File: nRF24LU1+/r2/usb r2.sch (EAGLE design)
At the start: 19 parts, among them IC2 NRF24L01SMD

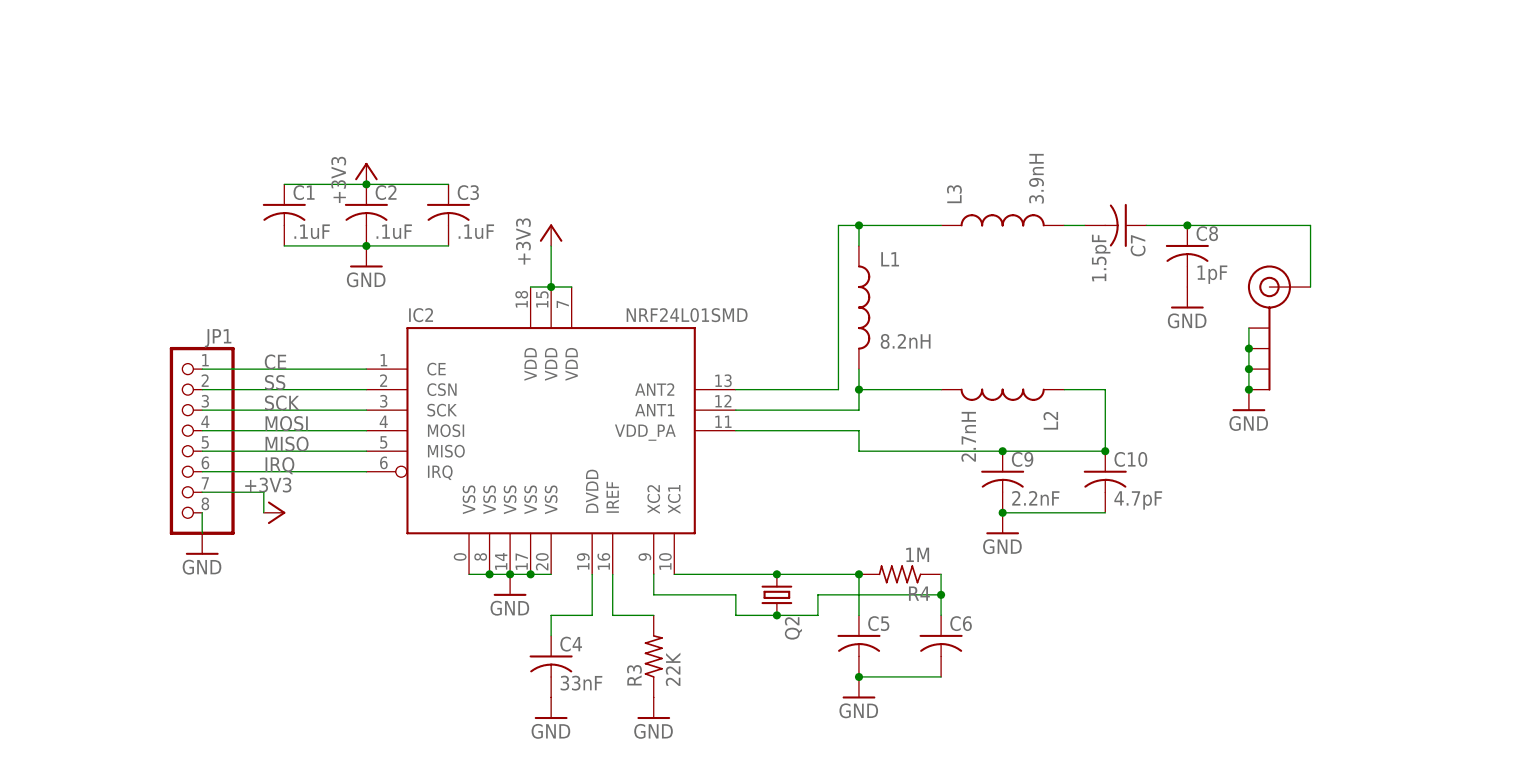
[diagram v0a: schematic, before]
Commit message: cleaning up, added a revised usb breakout
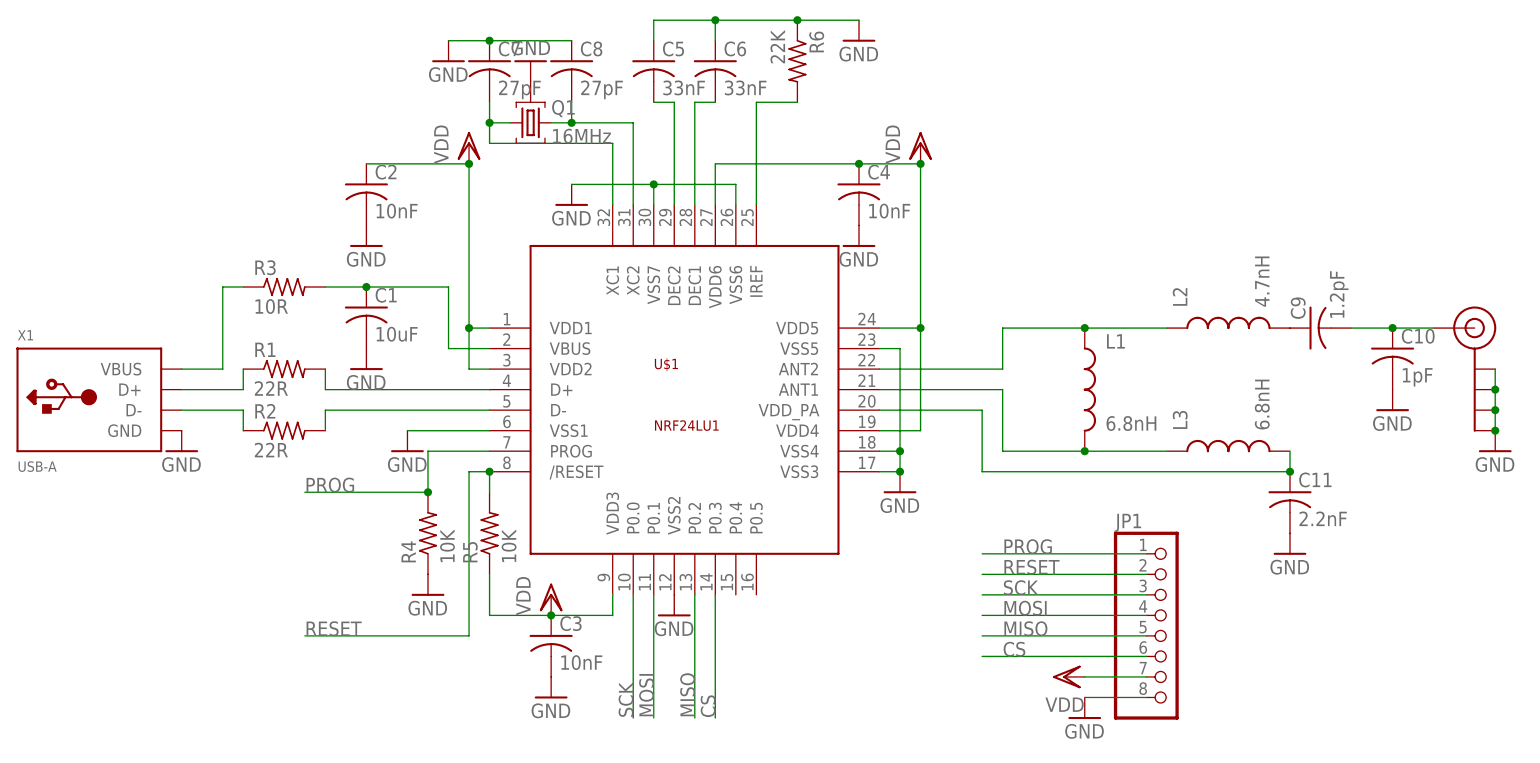
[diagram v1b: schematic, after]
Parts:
- removed IC2: NRF24L01SMD, SparkFun:NRF24L01SMD
- removed Q2: (no value), crystal:CRYSTALHC49U-V
- added C11: 2.2nF, adafruit:C-USC0402
- added Q1: 16MHz, crystal:TSX-3225
- added R1, R2: 22R, adafruit:R-US_R0402
- added R5: 10K, adafruit:R-US_R0402
- added R6: 22K, adafruit:R-US_R0402
- added U$1: NRF24LU1, SparkFun:NRF24LU1
- added X1: USB-A, adafruit:USB-A
- C1: value .1uF -> 10uF; device adafruit:C-USC0402 -> adafruit:C-USC0805K
- C10: value 4.7pF -> 1pF
- C2, C3: value .1uF -> 10nF
- C4: value 33nF -> 10nF
- C5, C6: value (none) -> 33nF
- C7: value 1.5pF -> 27pF
- C8: value 1pF -> 27pF
- C9: value 2.2nF -> 1.2pF
- L1: value 8.2nH -> 6.8nH
- L2: value 2.7nH -> 4.7nH
- L3: value 3.9nH -> 6.8nH
- R3: value 22K -> 10R
- R4: value 1M -> 10K
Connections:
- removed net +3V3: C1.1, C2.1, C3.1, IC2.VDD@15, IC2.VDD@18, IC2.VDD@7, JP1.7
- removed net CE: IC2.CE, JP1.1
- removed net IRQ: IC2.IRQ, JP1.6
- removed net N$17: C7.1, C8.1, J$1.SIGNAL
- removed net N$18: C10.1, C9.1, IC2.VDD_PA, L2.1
- removed net SS: IC2.CSN, JP1.2
- new net CS: JP1.6, U$1.P0.3
- new net N$1: R1.1, X1.D+
- new net N$2: R2.1, X1.D-
- new net N$3: R1.2, U$1.D+
- new net N$4: R2.2, U$1.D-
- new net N$5: C5.2, U$1.DEC2
- new net N$6: R3.1, X1.VBUS
- new net N$7: C1.1, R3.2, U$1.VBUS
- new net N$8: C6.2, U$1.DEC1
- new net N$9: R6.2, U$1.IREF
- new net PROG: JP1.1, R4.2, U$1.PROG
- new net RESET: JP1.2, R5.2, U$1./RESET
- new net VDD: C2.1, C3.1, C4.1, JP1.7, R5.1, U$1.VDD1, U$1.VDD2, U$1.VDD3, U$1.VDD4, U$1.VDD5, U$1.VDD6
- net GND: now also C11.2, C5.1, C6.1, C7.1, C8.1, Q1.3, R4.1, R6.1, U$1.VSS1, U$1.VSS2, U$1.VSS3, U$1.VSS4, U$1.VSS5, U$1.VSS6, U$1.VSS7, X1.GND; no longer C5.2, C6.2, C8.2, C9.2, IC2.VSS@0, IC2.VSS@14, IC2.VSS@17, IC2.VSS@20, IC2.VSS@8, R3.1
- net MISO: now also U$1.P0.2; no longer IC2.MISO
- net MOSI: now also U$1.P0.1; no longer IC2.MOSI
- net N$10: now also C8.2, Q1.2, U$1.XC2; no longer C4.1, IC2.DVDD
- net N$11: now also C7.2, Q1.1, U$1.XC1; no longer IC2.IREF, R3.2
- net N$12: now also C9.1, L2.2; no longer C5.1, IC2.XC1, Q2.1, R4.2
- net N$13: now also C10.1, C9.2, J$1.SIGNAL; no longer C6.1, IC2.XC2, Q2.2, R4.1
- net N$14: now also L2.1, U$1.ANT2; no longer IC2.ANT2, L3.1
- net N$15: now also C11.1, L3.2, U$1.VDD_PA; no longer IC2.ANT1, L1.2, L2.2
- net N$16: now also L1.2, L3.1, U$1.ANT1; no longer C7.2, L3.2
- net SCK: now also U$1.P0.0; no longer IC2.SCK
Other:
- moved on the sheet: C1, C10, C2, C3, C4, C5, C6, C7, C8, C9, JP1, L1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
